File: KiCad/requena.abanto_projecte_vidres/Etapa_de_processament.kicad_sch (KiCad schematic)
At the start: 15 parts, among them U1 PIC18F23K20_ISS, Y2 Crystal

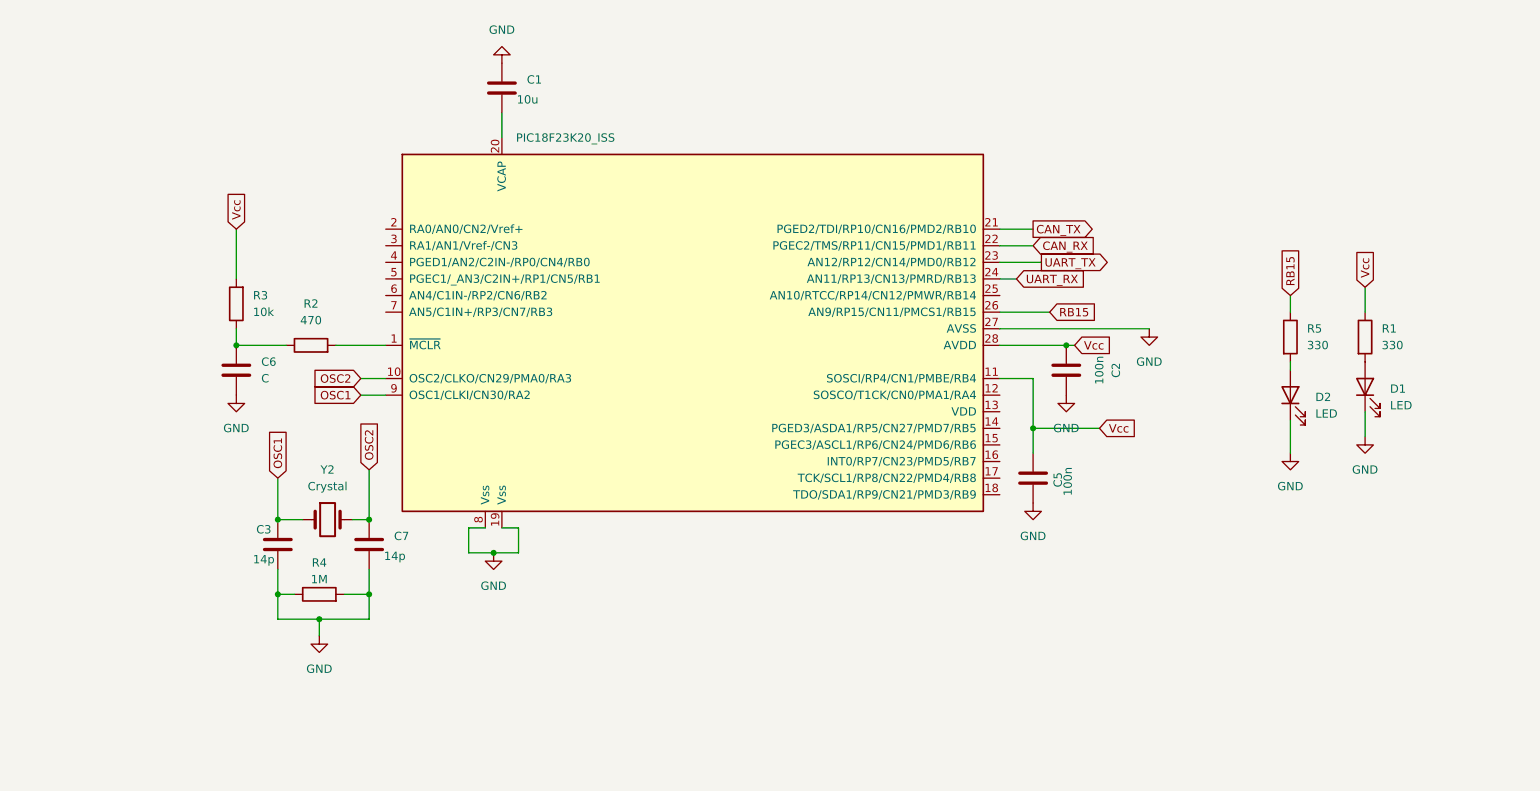
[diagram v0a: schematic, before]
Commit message: arreglos
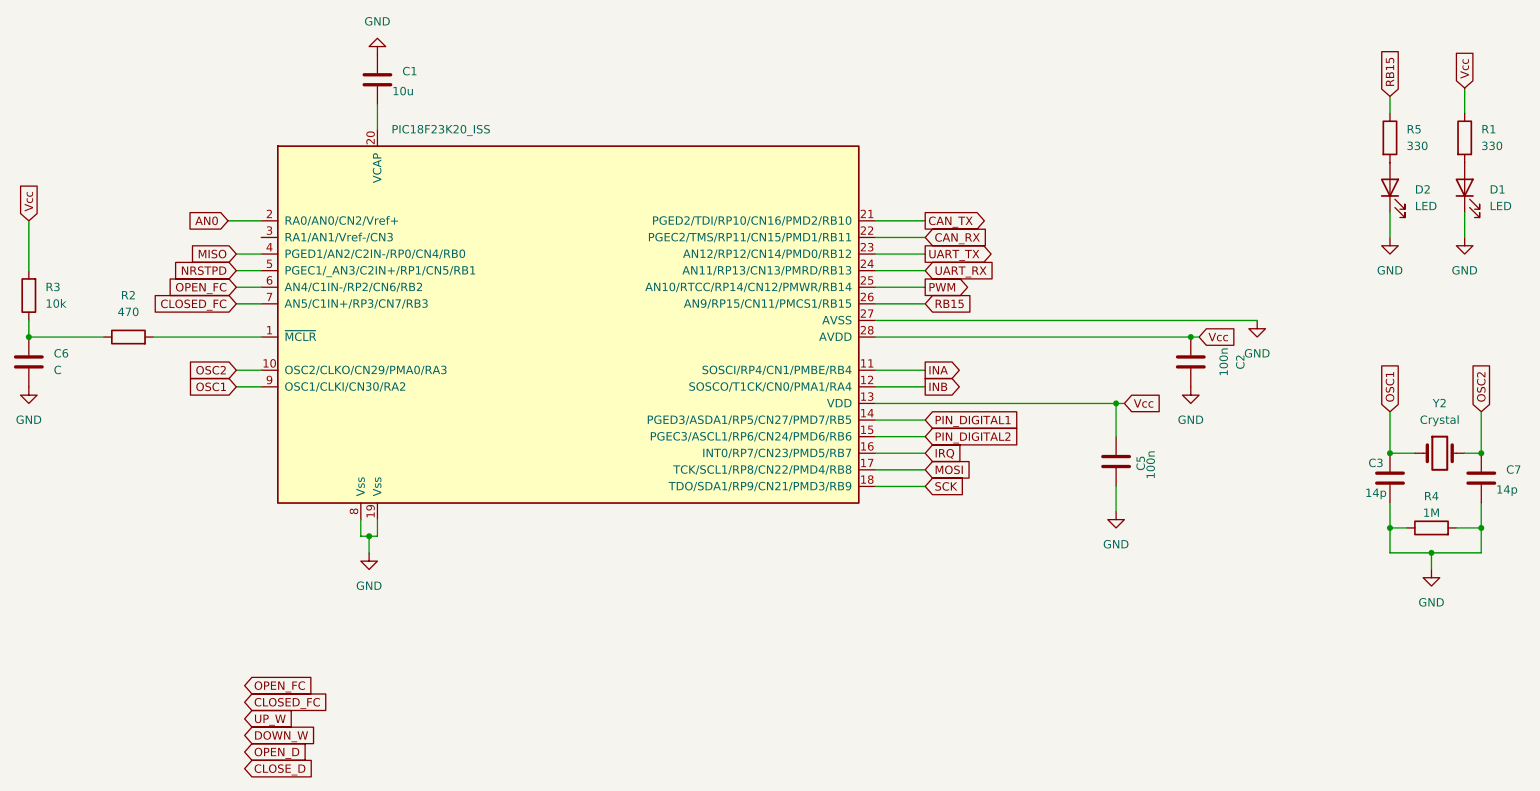
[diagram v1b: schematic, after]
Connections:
- net Vcc: now also U1.13 (VDD); no longer U1.11 (SOSCI/RP4/CN1/PMBE/RB4)
- net INB: now reaches U1.12 (SOSCO/T1CK/CN0/PMA1/RA4)
- net PIN_DIGITAL1: now reaches U1.14 (PGED3/ASDA1/RP5/CN27/PMD7/RB5)
- net PIN_DIGITAL2: now reaches U1.15 (PGEC3/ASCL1/RP6/CN24/PMD6/RB6)
- net IRQ: now reaches U1.16 (INT0/RP7/CN23/PMD5/RB7)
- net MOSI: now reaches U1.17 (TCK/SCL1/RP8/CN22/PMD4/RB8)
- net SCK: now reaches U1.18 (TDO/SDA1/RP9/CN21/PMD3/RB9)
- net AN0: now reaches U1.2 (RA0/AN0/CN2/Vref+)
- net PWM: now reaches U1.25 (AN10/RTCC/RP14/CN12/PMWR/RB14)
- net MISO: now reaches U1.4 (PGED1/AN2/C2IN-/RP0/CN4/RB0)
- net NRSTPD: now reaches U1.5 (PGEC1/_AN3/C2IN+/RP1/CN5/RB1)
- net OPEN_FC: now reaches U1.6 (AN4/C1IN-/RP2/CN6/RB2)
- net CLOSED_FC: now reaches U1.7 (AN5/C1IN+/RP3/CN7/RB3)
- new net INA: U1.11 (SOSCI/RP4/CN1/PMBE/RB4)
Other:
- moved on the sheet: C1, C2, C3, C5, C6, C7, D1, D2, R1, R2, R3, R4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
